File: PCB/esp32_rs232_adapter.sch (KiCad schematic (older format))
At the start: 8 parts

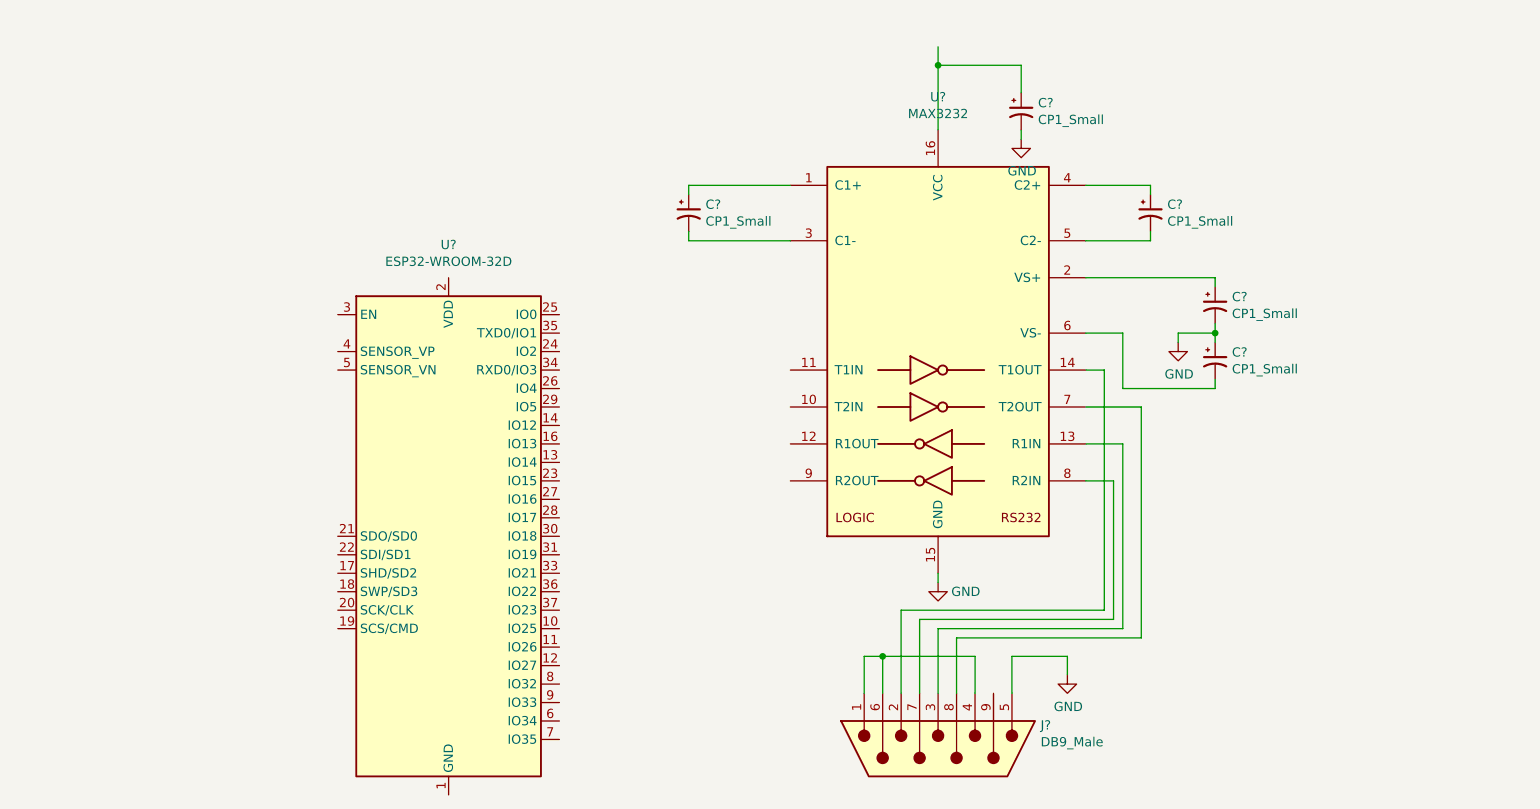
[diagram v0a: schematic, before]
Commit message: work on schematics
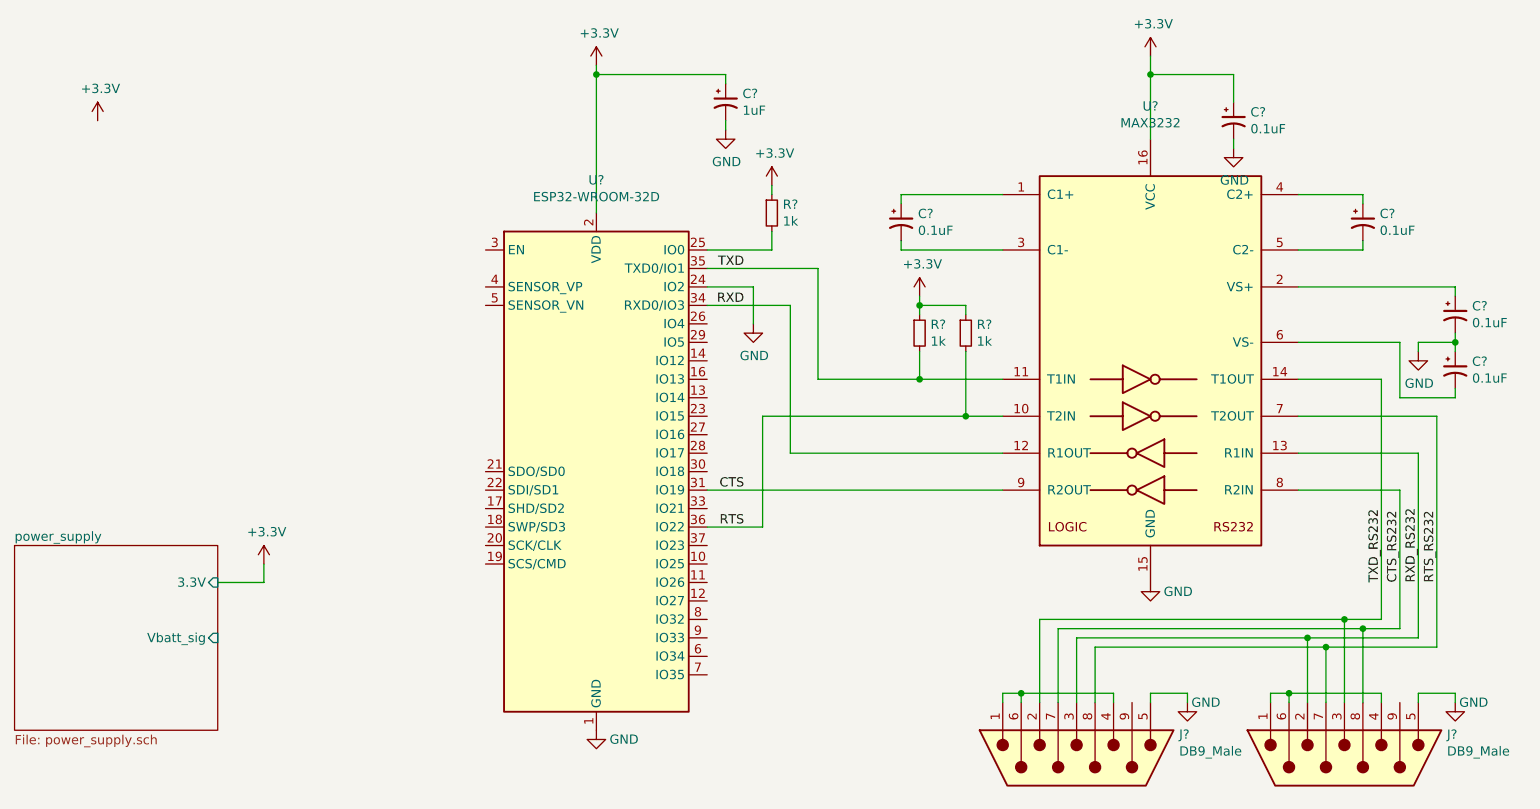
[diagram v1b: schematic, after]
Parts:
- removed C? (x4): CP1_Small, symbol Device:CP1_Small
- added C? (x4): 0.1uF, symbol Device:CP1_Small
- added C?: 1uF, symbol Device:CP1_Small
- added J?: DB9_Male, symbol Connector:DB9_Male
- added R? (x3): 1k, symbol Device:R_Small
- C?: value CP1_Small -> 0.1uF
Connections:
- net GND: now also U?.1 (GND), U?.15 (GND), U?.24 (IO2), U?.38 (GND), C?.1, C?.2, C?.2, C?.2, J?.5
- net RTS: now reaches U?.10 (T2IN)
- net RTS: now also U?.36 (IO22), R?.2
- net TXD: now reaches U?.11 (T1IN)
- net TXD: now also U?.35 (TXD0/IO1), R?.2
- net RXD: now reaches U?.12 (R1OUT)
- net RXD: now also U?.34 (RXD0/IO3)
- net RXD_RS232: now reaches J?.3, U?.13 (R1IN)
- net RXD_RS232: now also J?.2
- net TXD_RS232: now reaches J?.2, U?.14 (T1OUT)
- net TXD_RS232: now also J?.3
- net +3V3: now reaches U?.16 (VCC)
- net +3V3: now also U?.2 (VDD), C?.1, C?.1, R?.1, R?.1, R?.1
- net at U?.2 (VS+): now also C?.1
- net at U?.4 (C2+): now also C?.1
- net at U?.5 (C2-): now also C?.2
- net at U?.6 (VS-): now also C?.2
- net RTS_RS232: now reaches J?.8, U?.7 (T2OUT)
- net RTS_RS232: now also J?.7
- net CTS_RS232: now reaches J?.7, U?.8 (R2IN)
- net CTS_RS232: now also J?.8
- net CTS: now reaches U?.9 (R2OUT)
- net CTS: now also U?.31 (IO19)
- net at U?.25 (IO0): now also R?.2
- new net: J?.1, J?.4, J?.6
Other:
- moved on the sheet: C?, J?, U?
